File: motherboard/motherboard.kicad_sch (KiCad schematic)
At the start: 23 parts, among them J20 CM3588 Hirose Connector, J21 5V IN, J22 BATTERY IN, U26 AMS1117-1.8, U27 TPS54331DR

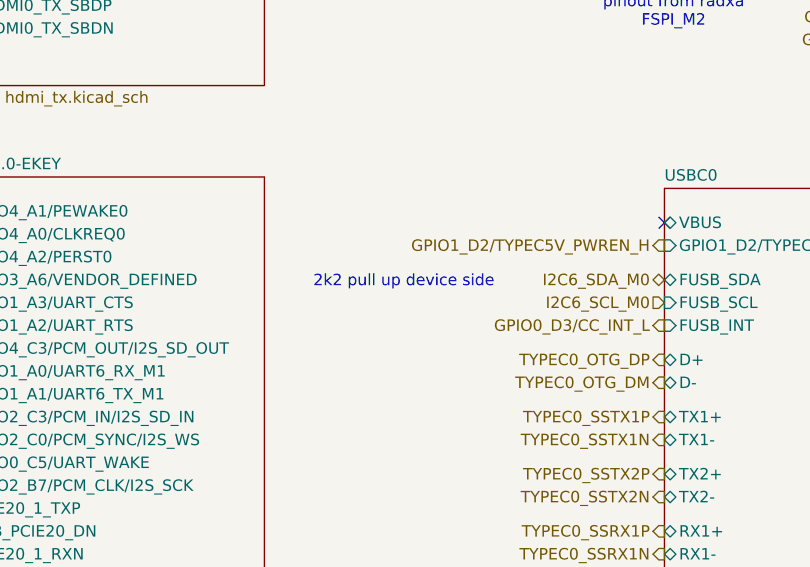
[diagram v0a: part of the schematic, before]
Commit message: layout nearing completion
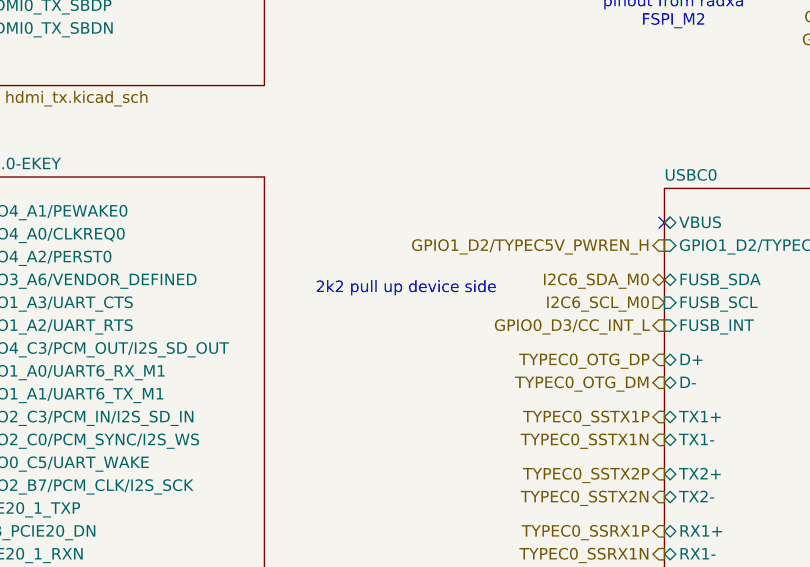
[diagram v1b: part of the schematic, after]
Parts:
- C80, C81, C83, C87, C88, C92, C93: footprint Capacitor_SMD:C_0402_1005Metric -> Capacitor_SMD:C_0603_1608Metric
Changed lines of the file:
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@@
 	(text "2k2 pull up device side"
 		(exclude_from_sim no)
-		(at 119.634 297.434 0)
+		(at 119.888 298.196 0)
 		(effects
 			(font
@@
 			)
 		)
-		(property "Footprint" "Capacitor_SMD:C_0402_1005Metric"
+		(property "Footprint" "Capacitor_SMD:C_0603_1608Metric"
 			(at 186.69 190.5 0)
 			(effects
@@
 			)
 		)
-		(property "Footprint" "Capacitor_SMD:C_0402_1005Metric"
+		(property "Footprint" "Capacitor_SMD:C_0603_1608Metric"
 			(at 373.38 200.66 0)
 			(effects
@@
 			)
 		)
-		(property "Footprint" "Capacitor_SMD:C_0402_1005Metric"
+		(property "Footprint" "Capacitor_SMD:C_0603_1608Metric"
 			(at 313.69 179.07 0)
 			(effects
@@
 			)
 		)
-		(property "Footprint" "Capacitor_SMD:C_0402_1005Metric"
+		(property "Footprint" "Capacitor_SMD:C_0603_1608Metric"
 			(at 420.37 212.09 0)
 			(effects
@@
 			)
 		)
-		(property "Footprint" "Capacitor_SMD:C_0402_1005Metric"
+		(property "Footprint" "Capacitor_SMD:C_0603_1608Metric"
 			(at 416.56 212.09 0)
 			(effects
@@
 			)
 		)
-		(property "Footprint" "Capacitor_SMD:C_0402_1005Metric"
+		(property "Footprint" "Capacitor_SMD:C_0603_1608Metric"
 			(at 334.01 179.07 0)
 			(effects
@@
 			)
 		)
-		(property "Footprint" "Capacitor_SMD:C_0402_1005Metric"
+		(property "Footprint" "Capacitor_SMD:C_0603_1608Metric"
 			(at 191.77 190.5 0)
 			(effects
